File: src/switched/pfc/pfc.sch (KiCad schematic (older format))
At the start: 67 parts, among them J1 AC-input, J2 Conn_01x02, J3 Conn_01x02, Q1 AOT190A60CL‎, U1 AP3917B, U2 bd7692fj

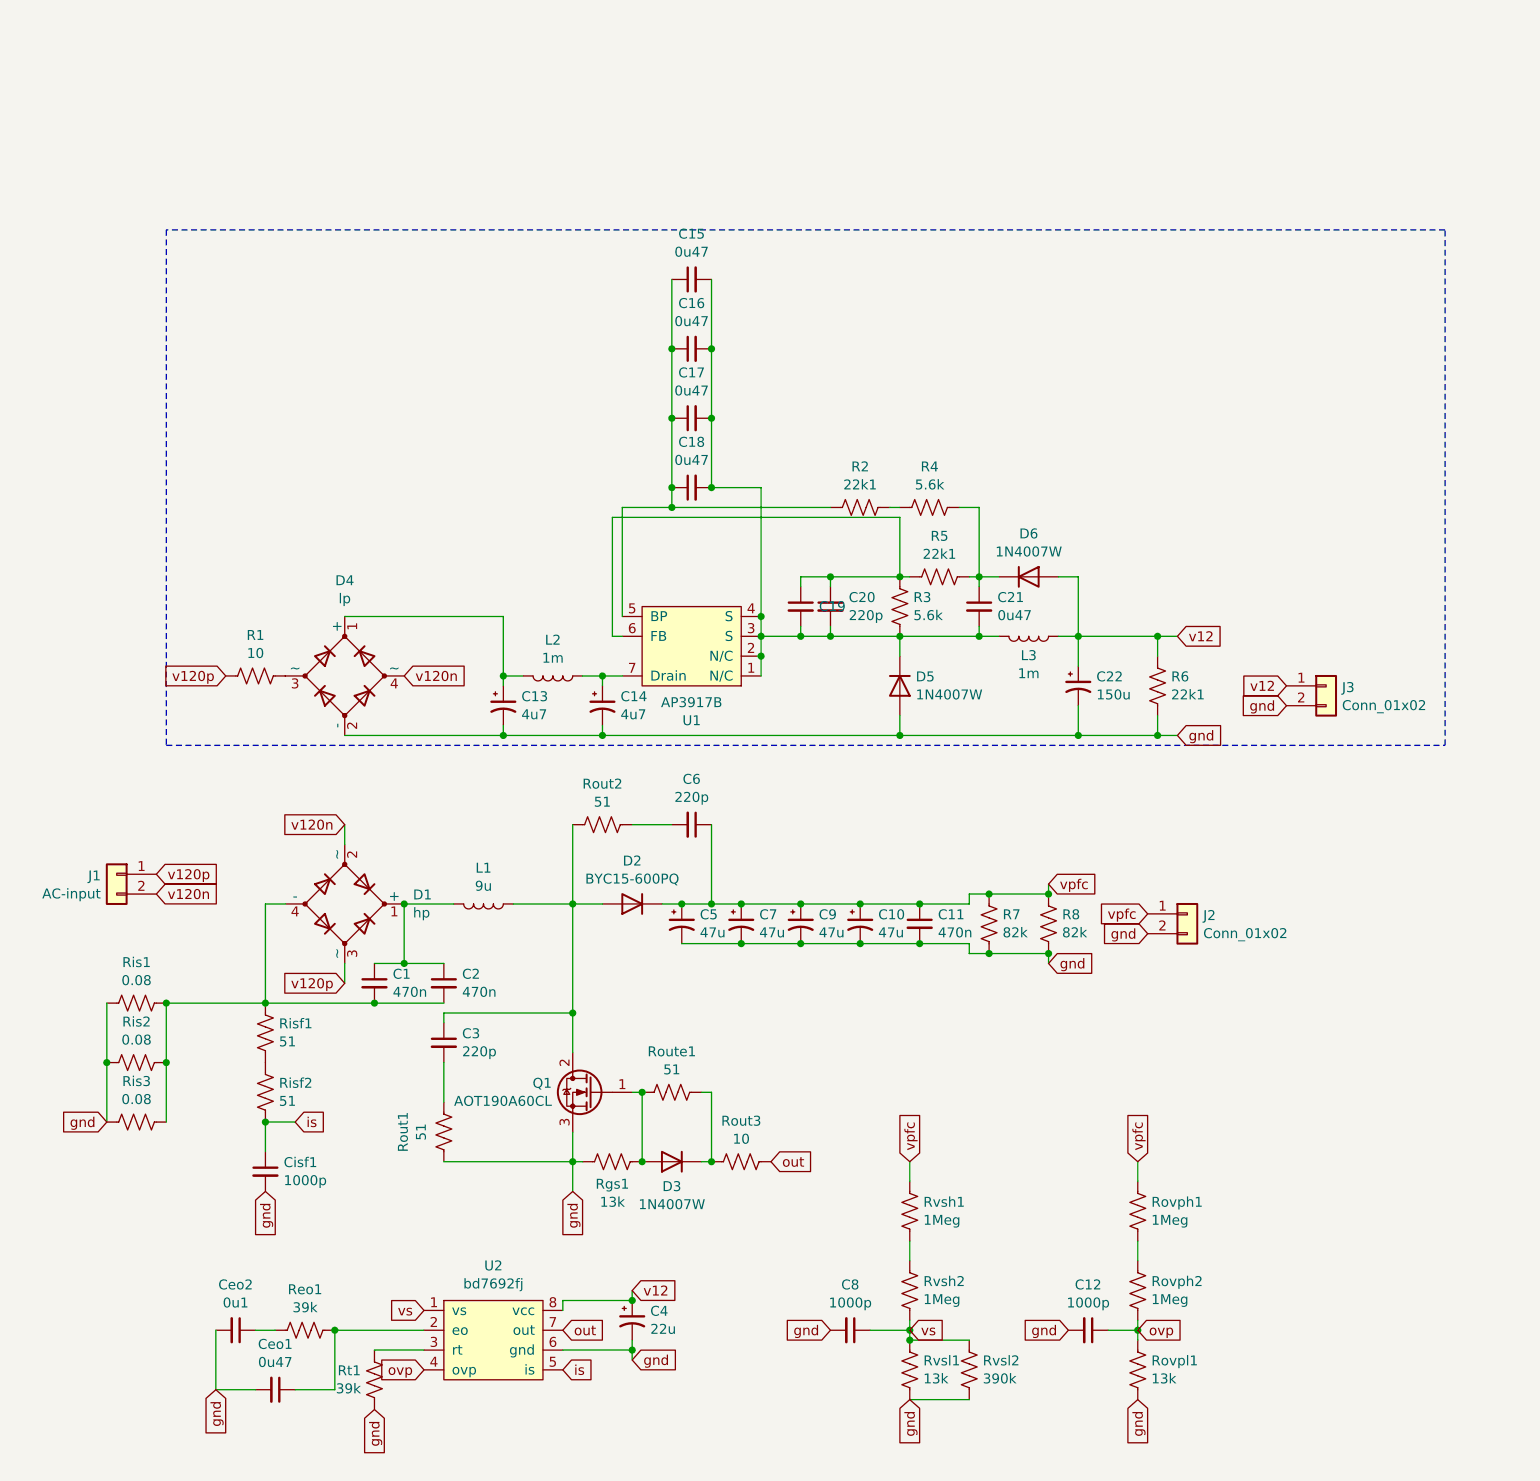
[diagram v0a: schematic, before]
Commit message: Midterm report
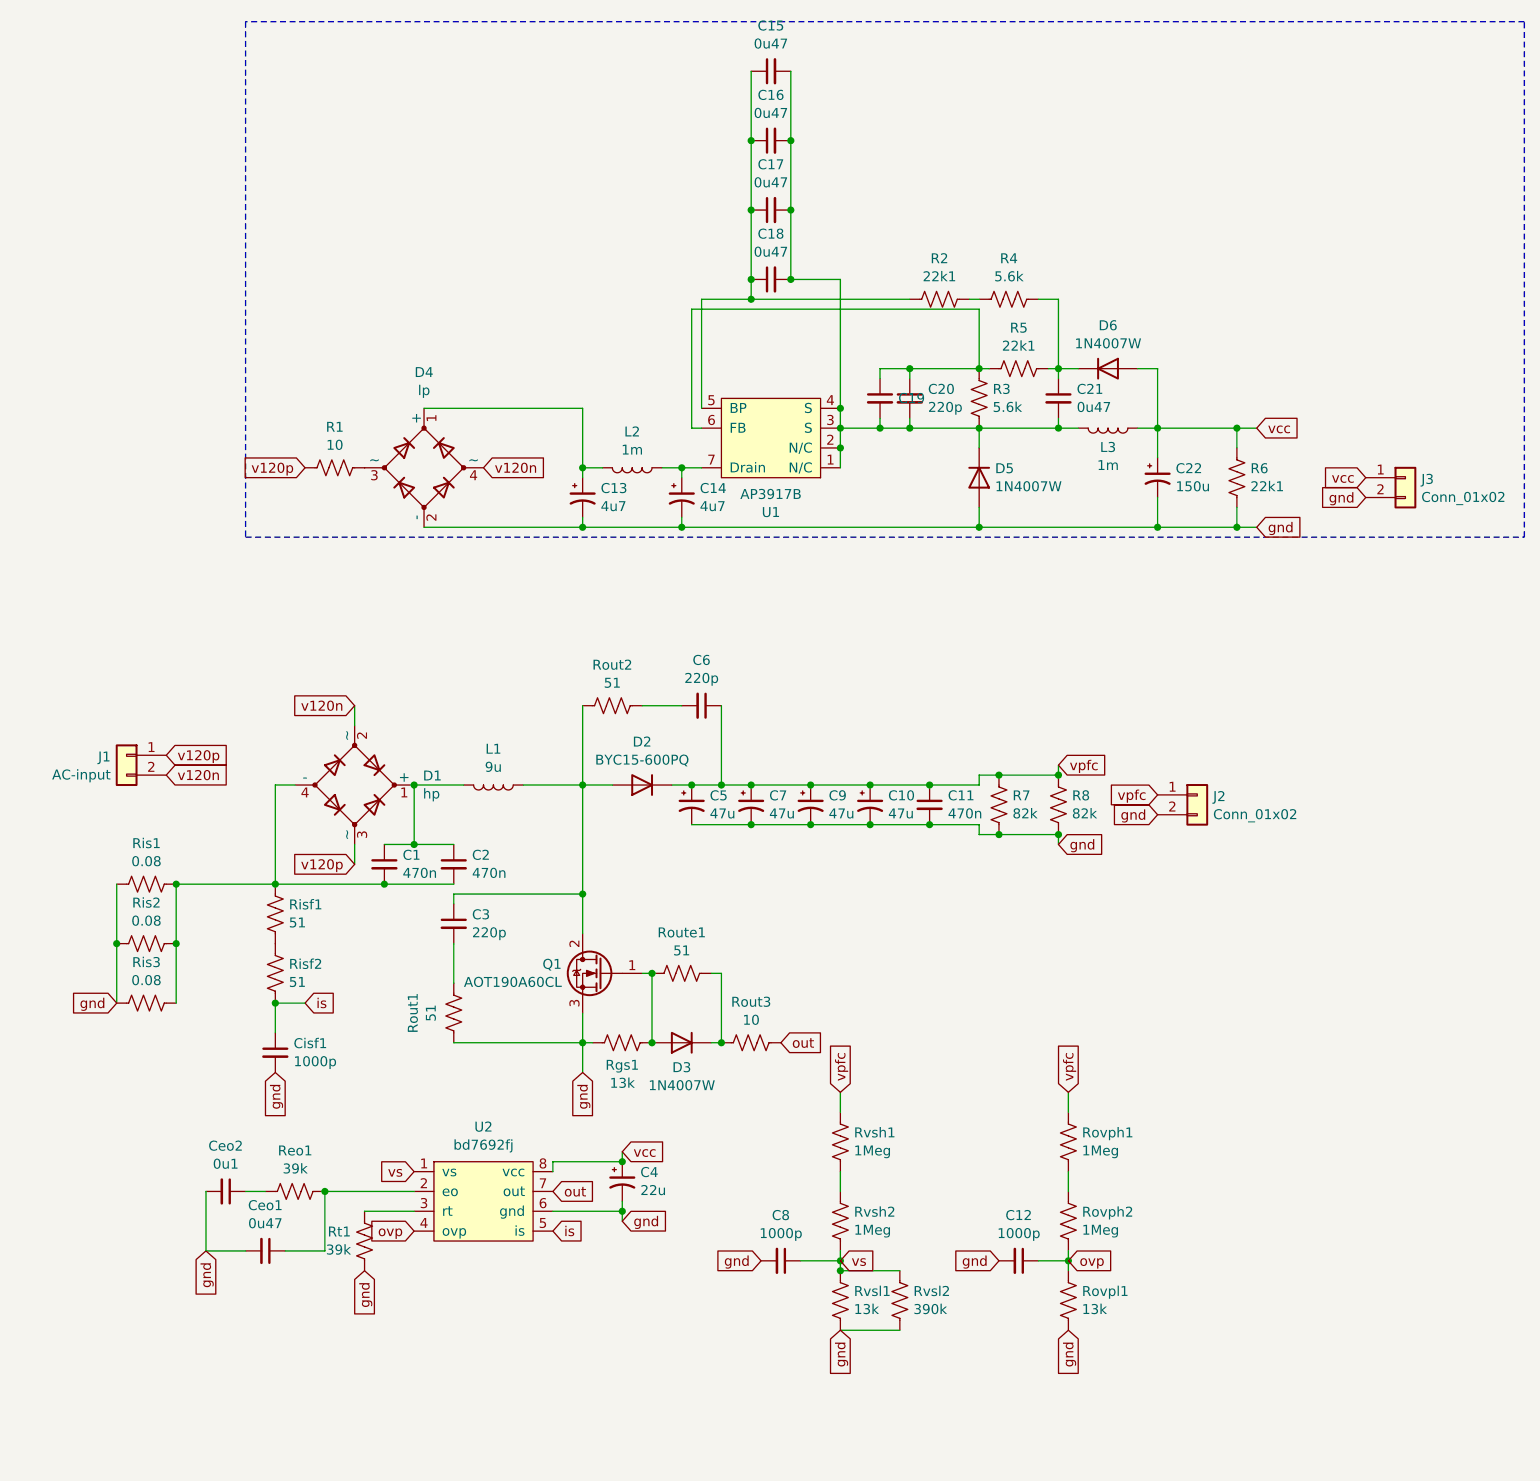
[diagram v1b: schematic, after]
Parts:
- C1, C11, C2: price 0.0143 -> 0.2238
- C10, C5, C7, C9: price 0.6115 -> 0.4815
- C12, C8, Cisf1: price 0.004 -> 0.0031
- C13, C14: price 0.039 -> 0.039
- C15, C16, C17, C18, C21, Ceo1: price 0.0143 -> 0.0112
- C19, C20, C3, C6: price 0.016 -> 0.0126
- C4: price 0.0125 -> 0.0098
- Ceo2: price 0.0041 -> 0.0032
- D1: price 0.6459 -> 0.5086
- D2: price 0.9091 -> 0.7159
- D3, D5, D6: price 0.0086 -> 0.0067
- D4: price 0.0342 -> 0.0271
- L2, L3: price 0.0974 -> 0.0772
- R1: price 0.0443 -> 0.0351
- R2, R5, R6: price 0.0041 -> 0.0041
- R3, R4: price 0.0087 -> 0.0052
- Reo1, Rt1: price 0.0091 -> 0.0071
- Rgs1, Rovpl1, Rvsl1, Rvsl2: price 0.0014 -> 0.0011
- Ris1, Ris2, Ris3: price 0.093 -> 0.0732
- Risf1, Risf2, Rout1, Rout2, Route1: price 0.0064 -> 0.005
- Rout3: price 0.0016 -> 0.0012
- Rovph1, Rovph2, Rvsh1, Rvsh2: price 0.0298 -> 0.0234
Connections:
- net v12 renamed vcc
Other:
- moved on the sheet: C1, C10, C11, C12, C13, C14, C15, C16, C17, C18, C19, C2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
